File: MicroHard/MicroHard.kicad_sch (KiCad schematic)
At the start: 0 parts

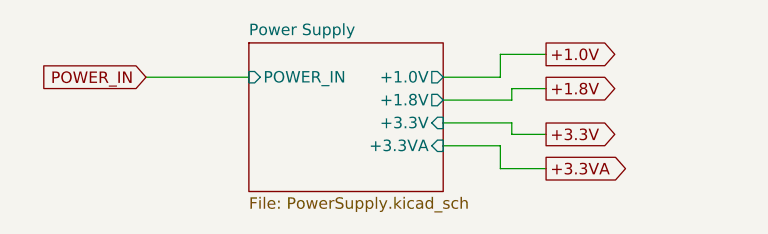
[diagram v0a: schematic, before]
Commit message: feat: added jumper
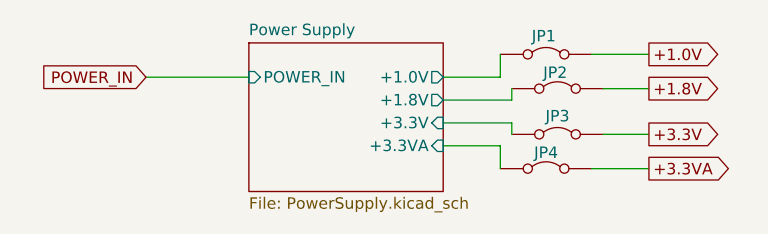
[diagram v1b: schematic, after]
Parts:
- added JP1, JP2, JP3, JP4: Jumper_2_Bridged, symbol Jumper:Jumper_2_Bridged
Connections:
- net +1.0V: now also JP1.2 (B)
- net +1.8V: now also JP2.2 (B)
- net +3.3V: now also JP3.2 (B)
- net +3.3VA: now also JP4.2 (B)
- new net Power Supply/+1.0V: JP1.1 (A)
- new net Power Supply/+1.8V: JP2.1 (A)
- new net Power Supply/+3.3V: JP3.1 (A)
- new net Power Supply/+3.3VA: JP4.1 (A)
